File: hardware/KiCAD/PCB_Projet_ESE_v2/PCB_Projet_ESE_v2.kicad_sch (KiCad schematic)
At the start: 101 parts, among them J1 Conn_01x06, J10 Conn_ST_STDC14, J2 Conn_01x06, J4 Conn_01x03, J5 Conn_01x04, J6 Conn_01x04, J9 Conn_01x02, SW4 SW_SPDT, SW5 SW_SPDT, U1 ZXBM5210-SP, U2 ZXBM5210-SP, U3 NCS210, U4 NCS210, U5 STM32G474RETx, U6 ADXL343, Y1 Crystal_GND24_Small

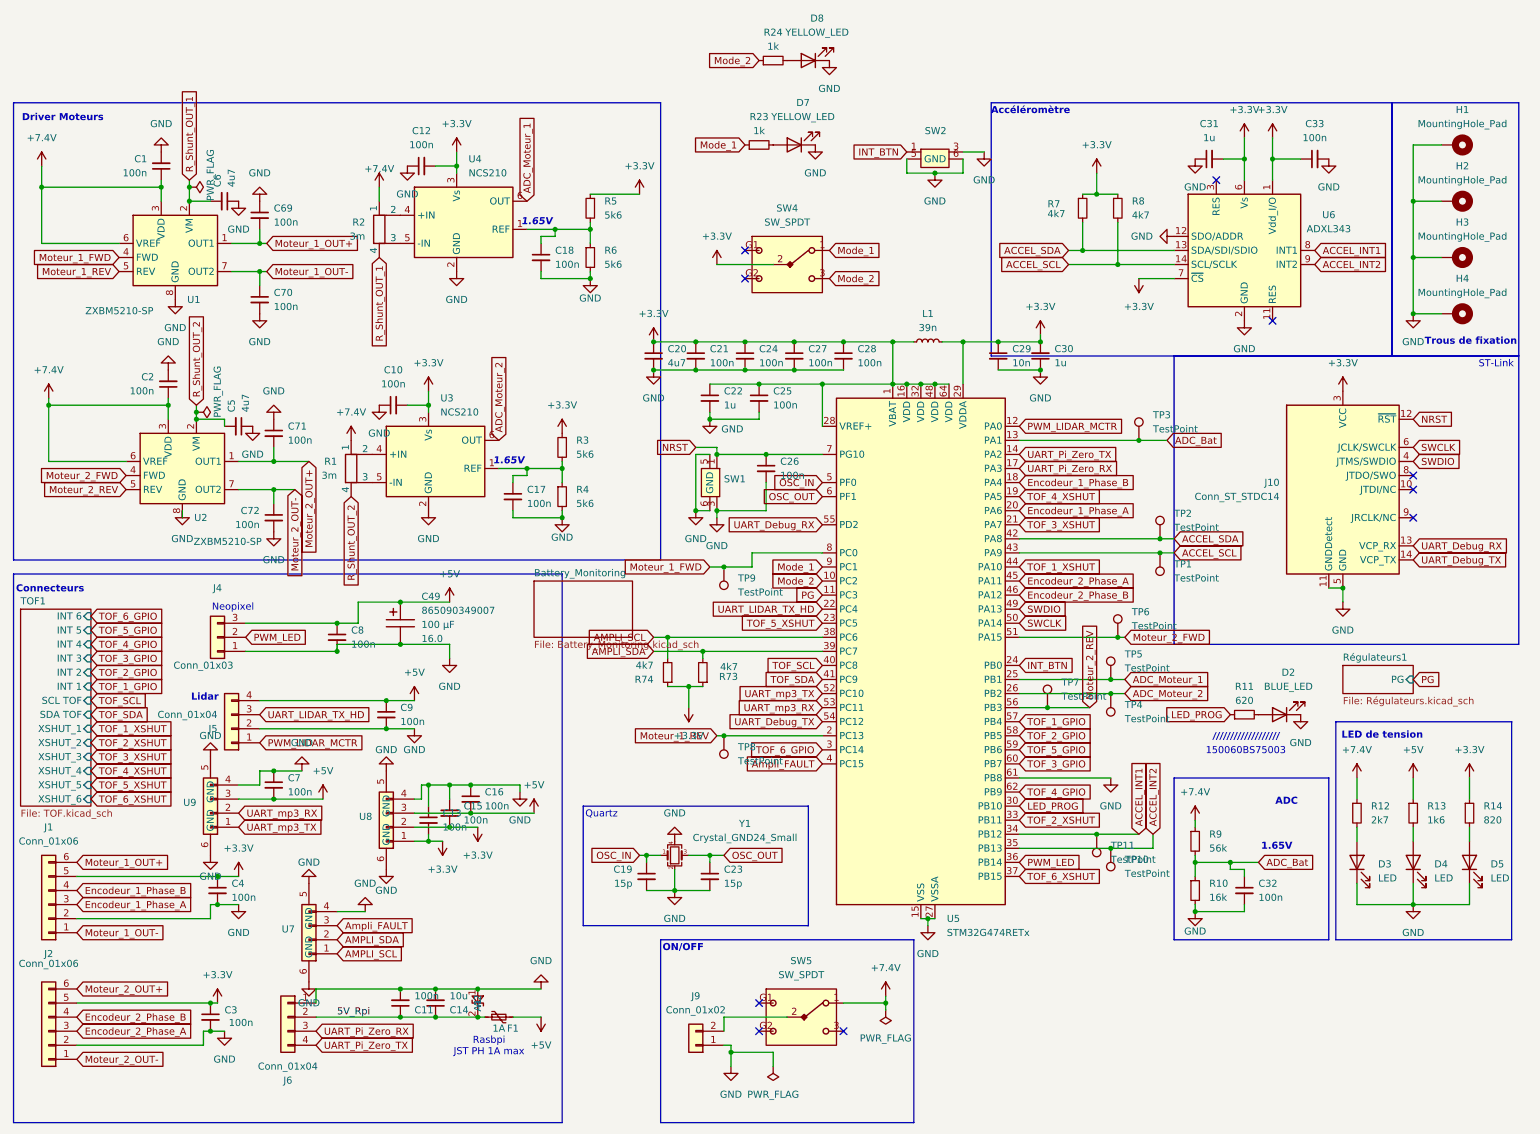
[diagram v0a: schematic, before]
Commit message: Finish README
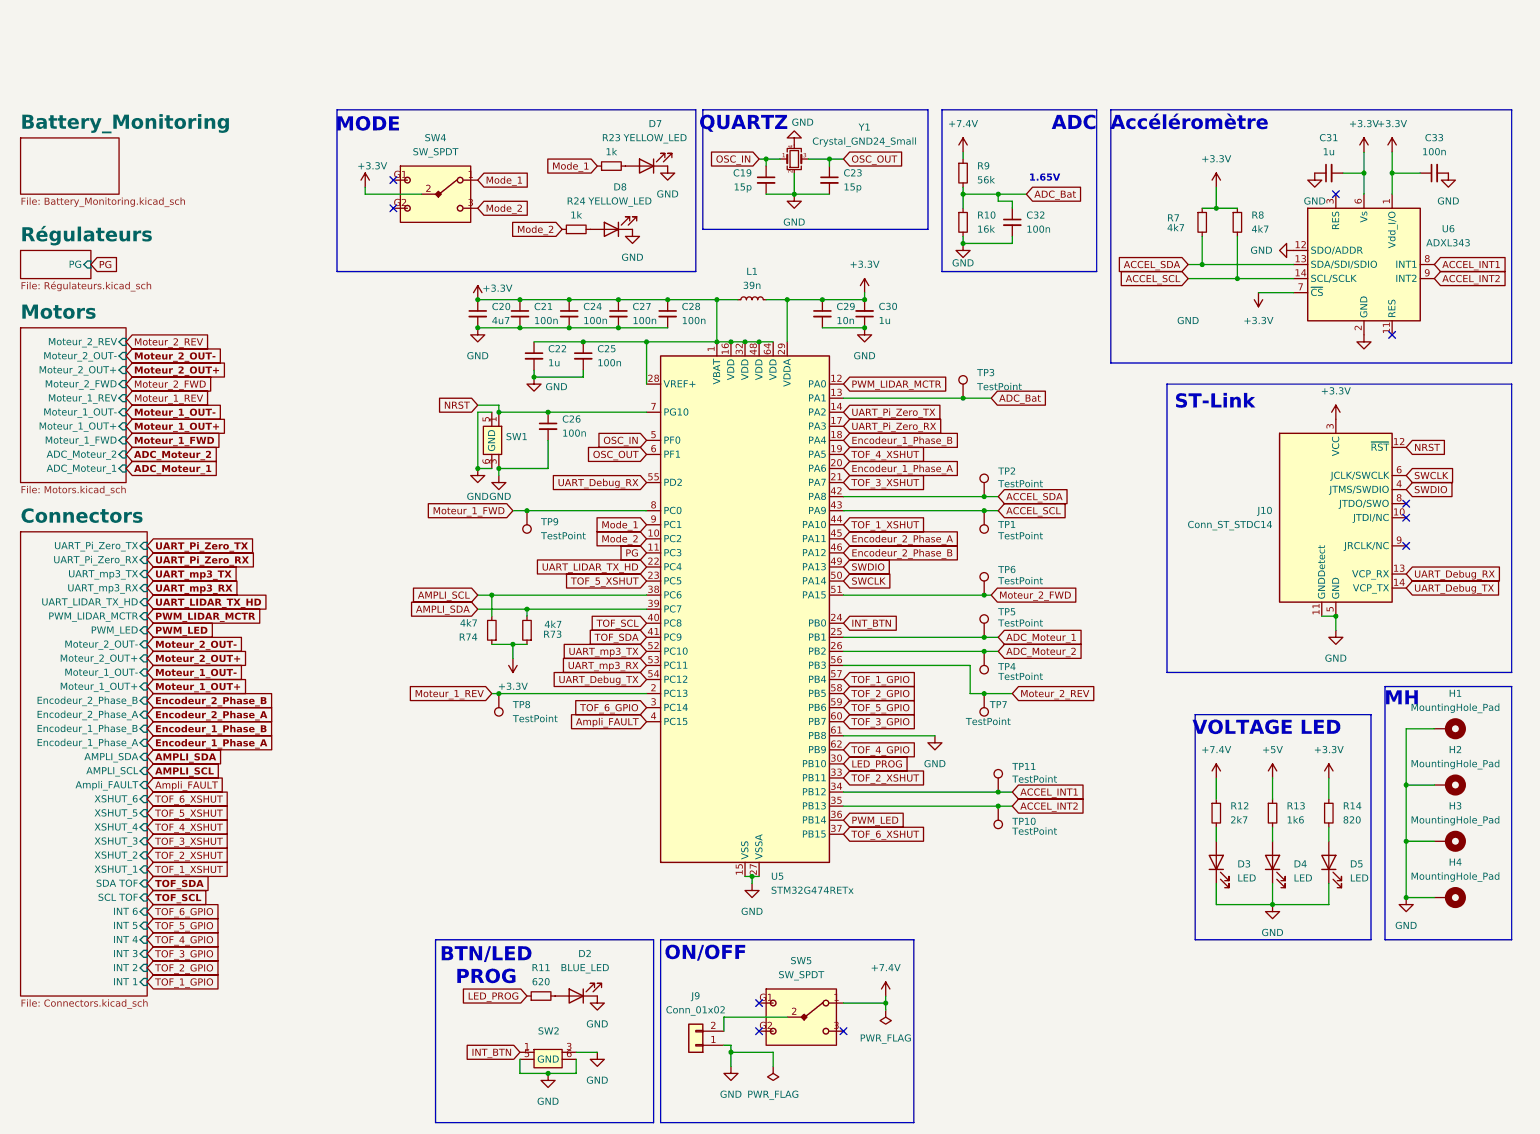
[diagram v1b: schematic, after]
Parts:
- removed C1, C10, C11, C12, C13, C15, C16, C17, C18, C2, C3, C4, C69, C7, C70, C71, C72, C8, C9: 100n, Capacitor_SMD:C_0402_1005Metric, symbol Device:C_Small
- removed C14: 10u, Capacitor_SMD:C_0603_1608Metric, symbol Device:C_Small
- removed C49: D8L6.5_865090349007, Capacitor_SMD_Wurth:CP_Wurth_WCAP-ASLU-D8L6.5, symbol Capacitor_Wurth_WCAP-ASLU:D8L6.5_865090349007
- removed C5, C6: 4u7, Capacitor_SMD:C_0603_1608Metric, symbol Device:C_Small
- removed D20: ~, Diode_SMD:D_SOD-523, symbol my_lib:VESD05A1-02V-G3-08
- removed F1: 1A, Fuse:Fuse_2920_7451Metric, symbol Device:Polyfuse_Small
- removed J1, J2: Conn_01x06, Connector_JST:JST_PH_S6B-PH-K_1x06_P2.00mm_Horizontal, symbol Connector_Generic:Conn_01x06
- removed J4: Conn_01x03, Connector_JST:JST_PH_B3B-PH-K_1x03_P2.00mm_Vertical, symbol Connector_Generic:Conn_01x03
- removed J5, J6: Conn_01x04, Connector_THT_Wurth:J_Wurth_WR-WTB_62000411722, symbol Connector_Generic:Conn_01x04
- removed R1, R2: 3m, Resistor_SMD:R_Shunt_Vishay_WSK2512_6332Metric_T2.21mm, symbol Device:R_Shunt
- removed R3, R4, R5, R6: 5k6, Resistor_SMD:R_0402_1005Metric, symbol Device:R_Small
- removed U1, U2: ZXBM5210-SP, Package_SO:Diodes_SO-8EP, symbol Driver_Motor:ZXBM5210-SP
- removed U3, U4: NCS210, Package_TO_SOT_SMD:SOT-363_SC-70-6, symbol Amplifier_Current:NCS210
- removed U7, U8, U9: ~, mylib:Wurth_Vertical_4_pos_0.8mm, symbol my_lib:JST_SH_4_Vertical
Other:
- sheet Régulateurs1 renamed Régulateurs
- removed sheet TOF1
- added sheet Connectors (Connectors.kicad_sch)
- added sheet Motors (Motors.kicad_sch)
- note added: "BTN/LED PROG"
- note added: "MH"
- note added: "MODE"
- note added: "QUARTZ"
- note added: "VOLTAGE LED"
- note removed: "///////////////////"
- note removed: "150060BS75003"
- note removed: "Connecteurs"
- note removed: "Driver Moteurs"
- note removed: "LED de tension"
- note removed: "Lidar"
- note removed: "Neopixel"
- note removed: "Quartz"
- note removed: "Rasbpi JST PH 1A max"
- note removed: "Trous de fixation"
- moved on the sheet: C19, C20, C21, C22, C23, C24, C25, C26, C27, C28, C29, C30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
